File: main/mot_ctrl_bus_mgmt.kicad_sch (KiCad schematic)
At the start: 20 parts, among them Q1601 IRLML0030, U1601 74LS08

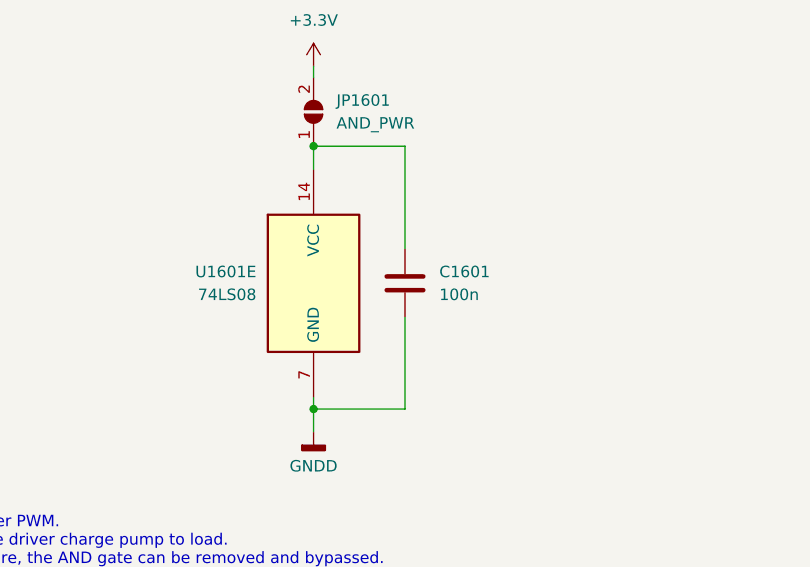
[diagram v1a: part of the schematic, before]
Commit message: Sent to fab
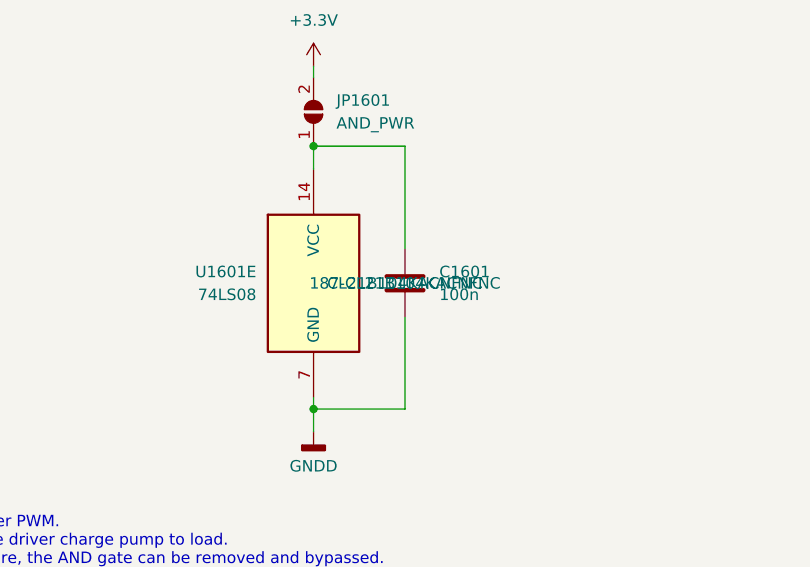
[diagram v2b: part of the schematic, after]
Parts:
- C1601: MPN (none) -> CL21B104KACNFNC; Mouser SKU (none) -> 187-CL21B104KACNFNC
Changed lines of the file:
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@@
+			)
+		)
+		(property "Quantity" ""
+			(at 231.14 48.26 0)
+			(effects
+				(font
+					(size 1.27 1.27)
+				)
 			)
 		)
@@
 			)
 		)
+		(property "Quantity" ""
+			(at 208.28 57.15 0)
+			(effects
+				(font
+					(size 1.27 1.27)
+				)
+			)
+		)
 		(pin "1"
 		)
@@
 			)
 		)
+		(property "Quantity" ""
+			(at 208.28 48.26 0)
+			(effects
+				(font
+					(size 1.27 1.27)
+				)
+			)
+		)
 		(pin "1"
 		)
@@
 			)
 		)
+		(property "Quantity" ""
+			(at 255.27 57.15 0)
+			(effects
+				(font
+					(size 1.27 1.27)
+				)
+			)
+		)
 		(pin "1"
 		)
@@
 				)
 				(hide yes)
+			)
+		)
+		(property "Quantity" ""
+			(at 219.71 57.15 0)
+			(effects
+				(font
+					(size 1.27 1.27)
+				)
 			)
 		)
@@
 			)
 		)
+		(property "Quantity" ""
+			(at 99.06 151.13 0)
+			(effects
+				(font
+					(size 1.27 1.27)
+				)
+			)
+		)
 		(pin "6"
 		)
@@
 			)
 		)
+		(property "Quantity" ""
+			(at 99.06 45.72 0)
+			(effects
+				(font
+					(size 1.27 1.27)
+				)
+			)
+		)
 		(pin "6"
 		)
@@
 			)
 		)
+		(property "Quantity" ""
+			(at 266.7 48.26 0)
+			(effects
+				(font
+					(size 1.27 1.27)
+				)
+			)
+		)
 		(pin "1"
 		)
@@
 			)
 		)
+		(property "MPN" "CL21B104KACNFNC "
+			(at 109.22 45.72 0)
+			(effects
+				(font
+					(size 1.27 1.27)
+				)
+			)
+		)
+		(property "Mouser SKU" " 187-CL21B104KACNFNC "
+			(at 109.22 45.72 0)
+			(effects
+				(font
+					(size 1.27 1.27)
+				)
+			)
+		)
+		(property "Quantity" ""
+			(at 109.22 45.72 0)
+			(effects
+				(font
+					(size 1.27 1.27)
+				)
+			)
+		)
 		(pin "1"
 		)
@@
 			)
 		)
+		(property "Quantity" ""
+			(at 99.06 100.33 0)
+			(effects
+				(font
+					(size 1.27 1.27)
+				)
+			)
+		)
 		(pin "6"
 		)
@@
 			)
 		)
+		(property "Quantity" ""
+			(at 109.22 93.98 0)
+			(effects
+				(font
+					(size 1.27 1.27)
+				)
+			)
+		)
 		(pin "2"
 		)
@@
 			)
 		)
+		(property "Quantity" ""
+			(at 250.19 81.28 0)
+			(effects
+				(font
+					(size 1.27 1.27)
+				)
+			)
+		)
 		(pin "2"
 		)
@@
 			)
 		)
+		(property "Quantity" ""
+			(at 243.84 57.15 0)
+			(effects
+				(font
+					(size 1.27 1.27)
+				)
+			)
+		)
 		(pin "1"
 		)
@@
 			)
 		)
+		(property "Quantity" ""
+			(at 109.22 119.38 0)
+			(effects
+				(font
+					(size 1.27 1.27)
+				)
+			)
+		)
 		(pin "2"
 		)
@@
 			)
 		)
+		(property "Quantity" ""
+			(at 109.22 144.78 0)
+			(effects
+				(font
+					(size 1.27 1.27)
+				)
+			)
+		)
 		(pin "2"
 		)
@@
 			)
 		)
+		(property "Quantity" ""
+			(at 99.06 26.67 0)
+			(effects
+				(font
+					(size 1.27 1.27)
+				)
+			)
+		)
 		(pin "2"
 		)
@@
 			)
 		)
+		(property "Quantity" ""
+			(at 231.14 57.15 0)
+			(effects
+				(font
+					(size 1.27 1.27)
+				)
+			)
+		)
 		(pin "1"
 		)
@@
 			)
 		)
+		(property "Quantity" ""
+			(at 266.7 57.15 0)
+			(effects
+				(font
+					(size 1.27 1.27)
+				)
+			)
+		)
 		(pin "1"
 		)
@@
 			)
 		)
+		(property "Quantity" ""
+			(at 99.06 171.45 0)
+			(effects
+				(font
+					(size 1.27 1.27)
+				)
+			)
+		)
 		(pin "6"
 		)
@@
 			)
 		)
+		(property "Quantity" ""
+			(at 255.27 48.26 0)
+			(effects
+				(font
+					(size 1.27 1.27)
+				)
+			)
+		)
 		(pin "1"
 		)
@@
 				)
 				(hide yes)
+			)
+		)
+		(property "Quantity" ""
+			(at 264.16 76.2 0)
+			(effects
+				(font
+					(size 1.27 1.27)
+				)
 			)
 		)
@@
 			)
 		)
+		(property "Quantity" ""
+			(at 99.06 125.73 0)
+			(effects
+				(font
+					(size 1.27 1.27)
+				)
+			)
+		)
 		(pin "6"
 		)
@@
 			)
 		)
+		(property "Quantity" ""
+			(at 243.84 48.26 0)
+			(effects
+				(font
+					(size 1.27 1.27)
+				)
+			)
+		)
 		(pin "1"
 		)
@@
 			)
 		)
+		(property "Quantity" ""
+			(at 219.71 48.26 0)
+			(effects
+				(font
+					(size 1.27 1.27)
+				)
+			)
+		)
